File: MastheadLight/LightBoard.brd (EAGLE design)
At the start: 7.6 x 22.9 mm, 6 parts, among them U1 WS2812, U2 WS2812

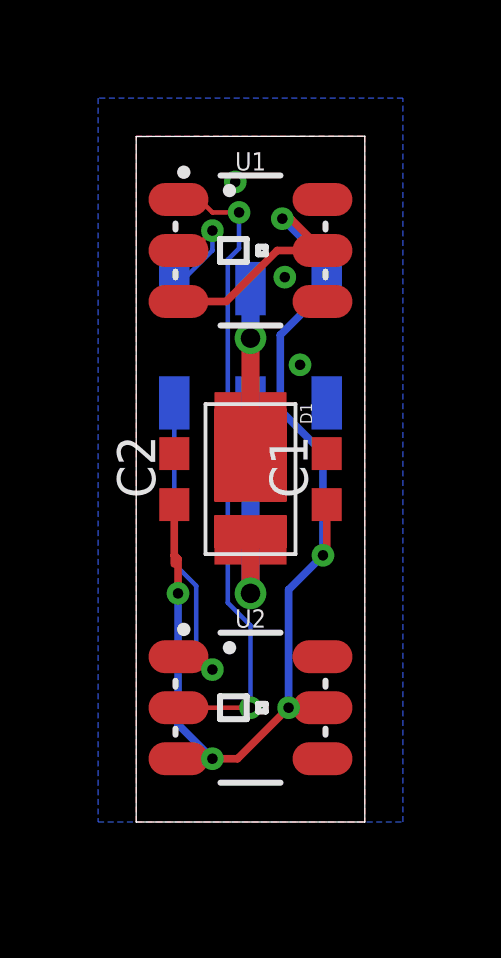
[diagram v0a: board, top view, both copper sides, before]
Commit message: As per Dec 2019 board orders
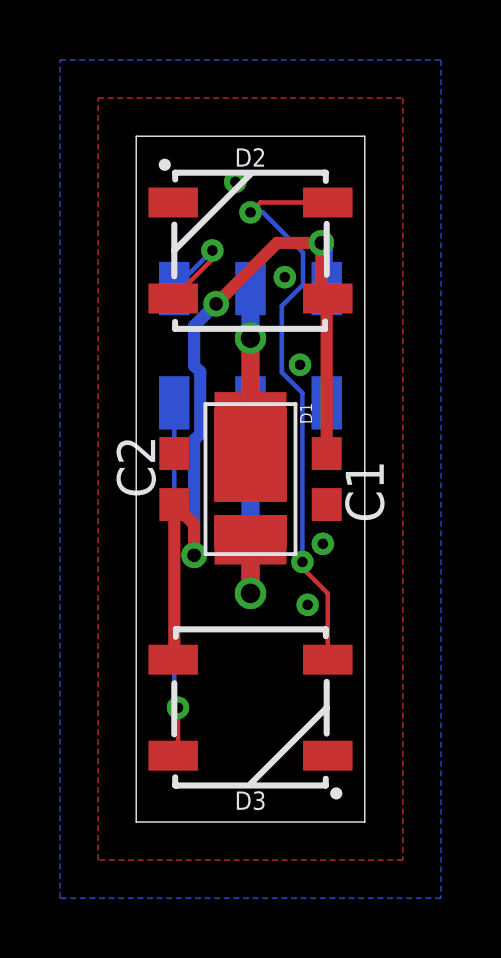
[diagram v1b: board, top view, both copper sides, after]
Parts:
- removed U1, U2: WS2812, SparkFun-LED:LED-TRICOLOR-5050-IC
- added D2, D3: WS2812B, SparkFun-LED:WS2812B
- turned C1 to 270 degrees
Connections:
- net +5V: now also D2.1, D3.1; no longer U1.3, U1.5, U2.3, U2.5
- net GND: now also D2.3, D3.3; no longer U1.6, U2.6
- net N$1: now also D2.2, D3.4; no longer U1.1, U2.2
- net N$2: now also D2.4; no longer U1.2
- net N$3: now also D3.2; no longer U2.1
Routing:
- net +5V: track 42.6 -> 29.1 mm, vias 5 -> 3
- net N$1: track 21.6 -> 19.5 mm
- net N$3: track 10.7 -> 11.9 mm
